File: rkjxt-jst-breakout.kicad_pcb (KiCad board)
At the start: 2 copper layers, 34 x 26.8 mm, 8 parts

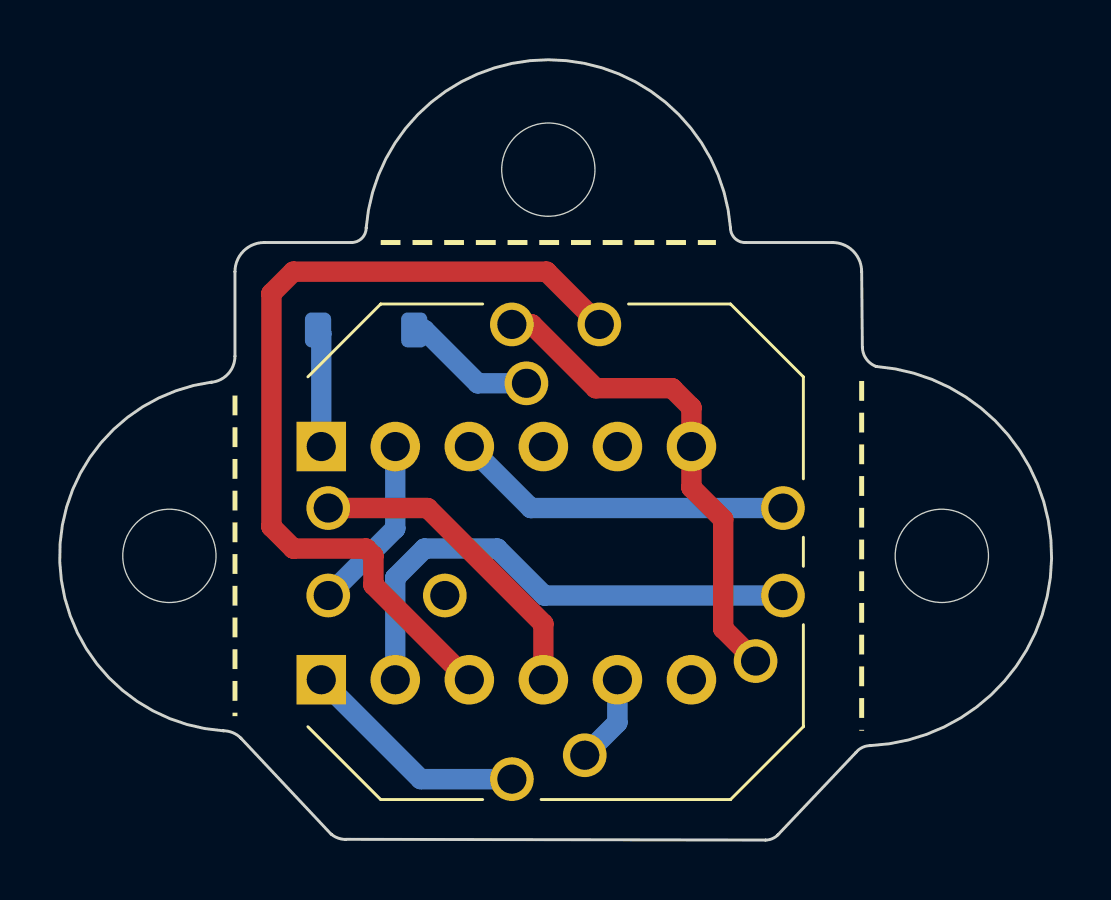
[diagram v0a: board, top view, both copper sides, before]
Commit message: fixing some issues, adding images
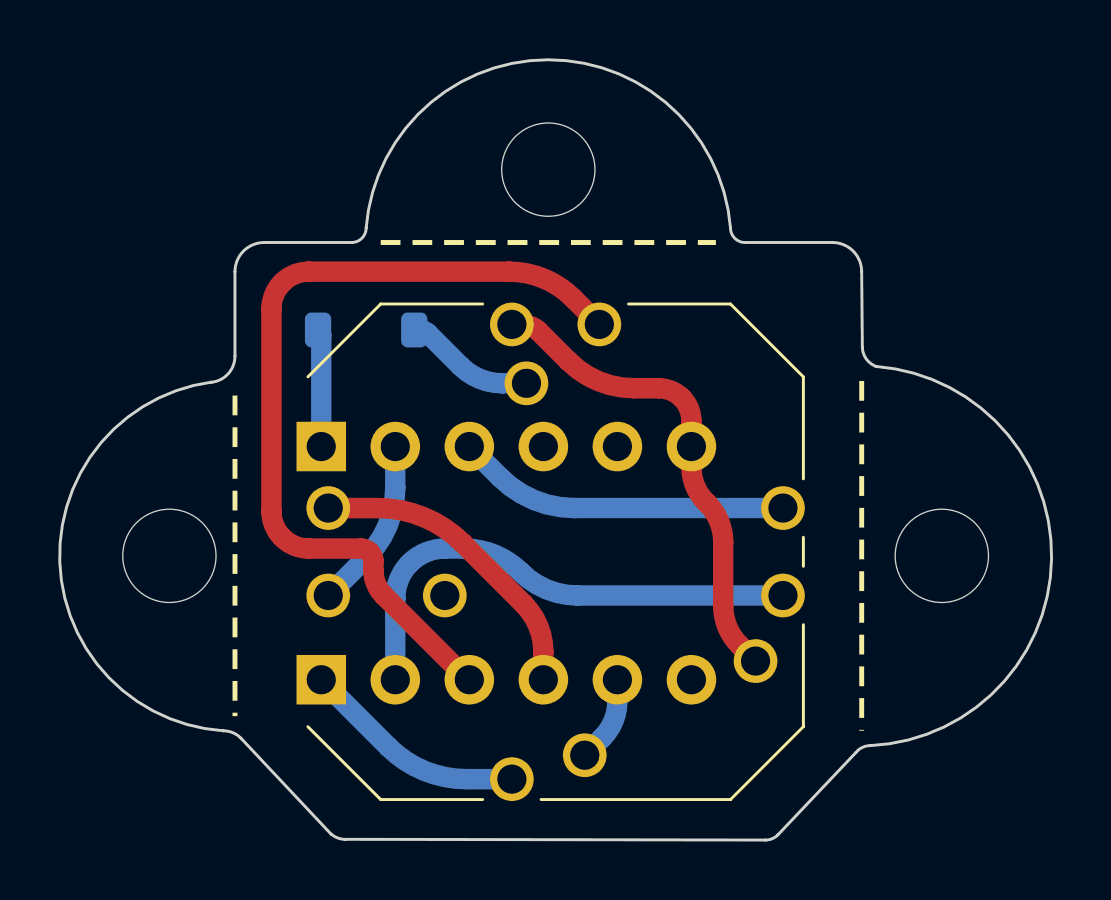
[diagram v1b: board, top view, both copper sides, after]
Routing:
- net Gnd: track 17.0 -> 16.4 mm
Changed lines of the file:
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@@
       (effects (font (size 1 1) (thickness 0.17) bold) (justify left top))
   )
-  (segment (start 134.96 75.11) (end 134.96 79) (width 0.7) (layer "B.Cu") (net 4))
-  (segment (start 134.85 75) (end 134.96 75.11) (width 0.7) (layer "B.Cu") (net 4))
-  (segment (start 140.33 76.83) (end 138.5 75) (width 0.7) (layer "B.Cu") (net 5))
-  (segment (start 138.5 75) (end 138.15 75) (width 0.7) (layer "B.Cu") (net 5))
-  (segment (start 142 76.83) (end 140.33 76.83) (width 0.7) (layer "B.Cu") (net 5))
-  (segment (start 145.12 88.47) (end 145.12 87) (width 0.7) (layer "B.Cu") (net 6))
-  (segment (start 144 89.59) (end 145.12 88.47) (width 0.7) (layer "B.Cu") (net 6))
-  (segment (start 142.58 85.08) (end 142.58 87) (width 0.7) (layer "F.Cu") (net 7))
-  (segment (start 138.61 81.11) (end 142.58 85.08) (width 0.7) (layer "F.Cu") (net 7))
-  (segment (start 135.2 81.11) (end 138.61 81.11) (width 0.7) (layer "F.Cu") (net 7))
-  (segment (start 133.25 81.75) (end 134 82.5) (width 0.7) (layer "F.Cu") (net 8))
-  (segment (start 144.5 74.81) (end 142.69 73) (width 0.7) (layer "F.Cu") (net 8))
-  (segment (start 134 73) (end 133.25 73.75) (width 0.7) (layer "F.Cu") (net 8))
-  (segment (start 136.75 83.75) (end 140 87) (width 0.7) (layer "F.Cu") (net 8))
-  (segment (start 136.5 82.5) (end 136.75 82.75) (width 0.7) (layer "F.Cu") (net 8))
-  (segment (start 133.25 73.75) (end 133.25 81.75) (width 0.7) (layer "F.Cu") (net 8))
-  (segment (start 142.69 73) (end 134 73) (width 0.7) (layer "F.Cu") (net 8))
-  (segment (start 136.75 82.75) (end 136.75 83.75) (width 0.7) (layer "F.Cu") (net 8))
-  (segment (start 134 82.5) (end 136.5 82.5) (width 0.7) (layer "F.Cu") (net 8))
-  (segment (start 140 87) (end 140.04 87) (width 0.7) (layer "F.Cu") (net 8))
-  (segment (start 138.5 82.5) (end 137.5 83.5) (width 0.7) (layer "B.Cu") (net 9))
-  (segment (start 137.5 83.5) (end 137.5 87) (width 0.7) (layer "B.Cu") (net 9))
-  (segment (start 141 82.5) (end 138.5 82.5) (width 0.7) (layer "B.Cu") (net 9))
-  (segment (start 150.8 84.11) (end 142.61 84.11) (width 0.7) (layer "B.Cu") (net 9))
-  (segment (start 142.61 84.11) (end 141 82.5) (width 0.7) (layer "B.Cu") (net 9))
-  (segment (start 141.5 90.41) (end 138.37 90.41) (width 0.7) (layer "B.Cu") (net 10))
-  (segment (start 138.37 90.41) (end 134.96 87) (width 0.7) (layer "B.Cu") (net 10))
-  (segment (start 137.5 81.81) (end 135.2 84.11) (width 0.7) (layer "B.Cu") (net 11))
-  (segment (start 137.5 79) (end 137.5 81.81) (width 0.7) (layer "B.Cu") (net 11))
-  (segment (start 142.15 81.11) (end 140.04 79) (width 0.7) (layer "B.Cu") (net 12))
-  (segment (start 150.8 81.11) (end 142.15 81.11) (width 0.7) (layer "B.Cu") (net 12))
-  (segment (start 147 77) (end 144.375 77) (width 0.7) (layer "F.Cu") (net 13))
-  (segment (start 147.66 77.66) (end 147 77) (width 0.7) (layer "F.Cu") (net 13))
-  (segment (start 142.185 74.81) (end 141.5 74.81) (width 0.7) (layer "F.Cu") (net 13))
-  (segment (start 147.66 80.41) (end 147.66 79) (width 0.7) (layer "F.Cu") (net 13))
-  (segment (start 147.66 79) (end 147.66 77.66) (width 0.7) (layer "F.Cu") (net 13))
-  (segment (start 149.86 86.36) (end 148.75 85.25) (width 0.7) (layer "F.Cu") (net 13))
-  (segment (start 148.75 85.25) (end 148.75 81.5) (width 0.7) (layer "F.Cu") (net 13))
-  (segment (start 148.75 81.5) (end 147.66 80.41) (width 0.7) (layer "F.Cu") (net 13))
-  (segment (start 144.375 77) (end 142.185 74.81) (width 0.7) (layer "F.Cu") (net 13))
+  (segment (start 134.96 75.187781) (end 134.96 79) (width 0.7) (layer "B.Cu") (net 4))
+  (segment (start 134.905 75.055) (end 134.85 75) (width 0.7) (layer "B.Cu") (net 4))
+  (arc (start 134.905 75.055) (mid 134.945705 75.11592) (end 134.96 75.187781) (width 0.7) (layer "B.Cu") (net 4))
+  (segment (start 138.623743 75.123743) (end 139.739565 76.239565) (width 0.7) (layer "B.Cu") (net 5))
+  (segment (start 138.325 75) (end 138.15 75) (width 0.7) (layer "B.Cu") (net 5))
+  (segment (start 141.165 76.83) (end 142 76.83) (width 0.7) (layer "B.Cu") (net 5))
+  (arc (start 139.739565 76.239565) (mid 140.39356 76.67655) (end 141.165 76.83) (width 0.7) (layer "B.Cu") (net 5))
+  (arc (start 138.623743 75.123743) (mid 138.486678 75.032159) (end 138.325 75) (width 0.7) (layer "B.Cu") (net 5))
+  (segment (start 145.12 87.735) (end 145.12 87) (width 0.7) (layer "B.Cu") (net 6))
+  (segment (start 144.600276 88.989723) (end 144 89.59) (width 0.7) (layer "B.Cu") (net 6))
+  (arc (start 145.12 87.735) (mid 144.984928 88.414051) (end 144.600276 88.989723) (width 0.7) (layer "B.Cu") (net 6))
+  (segment (start 142.58 86.04) (end 142.58 87) (width 0.7) (layer "F.Cu") (net 7))
+  (segment (start 141.901177 84.401177) (end 139.815617 82.315617) (width 0.7) (layer "F.Cu") (net 7))
+  (segment (start 136.905 81.11) (end 135.2 81.11) (width 0.7) (layer "F.Cu") (net 7))
+  (arc (start 139.815617 82.315617) (mid 138.480214 81.423329) (end 136.905 81.11) (width 0.7) (layer "F.Cu") (net 7))
+  (arc (start 141.901177 84.401177) (mid 142.403579 85.153075) (end 142.58 86.04) (width 0.7) (layer "F.Cu") (net 7))
+  (segment (start 143.595 73.905) (end 144.5 74.81) (width 0.7) (layer "F.Cu") (net 8))
+  (segment (start 137.103553 84.103553) (end 139.985857 86.985857) (width 0.7) (layer "F.Cu") (net 8))
+  (segment (start 133.25 81.219669) (end 133.25 74.28033) (width 0.7) (layer "F.Cu") (net 8))
+  (segment (start 141.410136 73) (end 134.53033 73) (width 0.7) (layer "F.Cu") (net 8))
+  (segment (start 136.75 83.25) (end 136.75 82.926776) (width 0.7) (layer "F.Cu") (net 8))
+  (segment (start 136.323223 82.5) (end 134.53033 82.5) (width 0.7) (layer "F.Cu") (net 8))
+  (segment (start 140.02 87) (end 140.04 87) (width 0.7) (layer "F.Cu") (net 8))
+  (arc (start 136.625 82.625) (mid 136.717513 82.763456) (end 136.75 82.926776) (width 0.7) (layer "F.Cu") (net 8))
+  (arc (start 143.595 73.905) (mid 142.592576 73.235201) (end 141.410136 73) (width 0.7) (layer "F.Cu") (net 8))
+  (arc (start 136.75 83.25) (mid 136.841885 83.711939) (end 137.103553 84.103553) (width 0.7) (layer "F.Cu") (net 8))
+  (arc (start 133.25 81.219669) (mid 133.347459 81.70963) (end 133.625 82.125) (width 0.7) (layer "F.Cu") (net 8))
+  (arc (start 139.985857 86.985857) (mid 140.001522 86.996324) (end 140.02 87) (width 0.7) (layer "F.Cu") (net 8))
+  (arc (start 134.53033 73) (mid 134.040368 73.097459) (end 133.625 73.375) (width 0.7) (layer "F.Cu") (net 8))
+  (arc (start 133.625 82.125) (mid 134.040368 82.40254) (end 134.53033 82.5) (width 0.7) (layer "F.Cu") (net 8))
+  (arc (start 136.625 82.625) (mid 136.486543 82.532486) (end 136.323223 82.5) (width 0.7) (layer "F.Cu") (net 8))
+  (arc (start 133.625 73.375) (mid 133.347459 73.790368) (end 133.25 74.28033) (width 0.7) (layer "F.Cu") (net 8))
+  (segment (start 137.5 84.207106) (end 137.5 87) (width 0.7) (layer "B.Cu") (net 9))
+  (segment (start 139.861558 82.5) (end 139.207106 82.5) (width 0.7) (layer "B.Cu") (net 9))
+  (segment (start 143.748441 84.11) (end 150.8 84.11) (width 0.7) (layer "B.Cu") (net 9))
+  (arc (start 141.805 83.305) (mid 140.913341 82.709212) (end 139.861558 82.5) (width 0.7) (layer "B.Cu") (net 9))
+  (arc (start 139.207106 82.5) (mid 138.553825 82.629945) (end 138 83) (width 0.7) (layer "B.Cu") (net 9))
+  (arc (start 141.805 83.305) (mid 142.696658 83.900787) (end 143.748441 84.11) (width 0.7) (layer "B.Cu") (net 9))
+  (arc (start 138 83) (mid 137.629945 83.553825) (end 137.5 84.207106) (width 0.7) (layer "B.Cu") (net 9))
+  (segment (start 139.935 90.41) (end 141.5 90.41) (width 0.7) (layer "B.Cu") (net 10))
+  (segment (start 137.263377 89.303377) (end 134.96 87) (width 0.7) (layer "B.Cu") (net 10))
+  (arc (start 137.263377 89.303377) (mid 138.489128 90.122398) (end 139.935 90.41) (width 0.7) (layer "B.Cu") (net 10))
+  (segment (start 136.506514 82.803485) (end 135.2 84.11) (width 0.7) (layer "B.Cu") (net 11))
+  (segment (start 137.5 80.405) (end 137.5 79) (width 0.7) (layer "B.Cu") (net 11))
+  (arc (start 137.5 80.405) (mid 137.241801 81.70305) (end 136.506514 82.803485) (width 0.7) (layer "B.Cu") (net 11))
+  (segment (start 141.095 80.055) (end 140.04 79) (width 0.7) (layer "B.Cu") (net 12))
+  (segment (start 143.641995 81.11) (end 150.8 81.11) (width 0.7) (layer "B.Cu") (net 12))
+  (arc (start 141.095 80.055) (mid 142.263571 80.835814) (end 143.641995 81.11) (width 0.7) (layer "B.Cu") (net 12))
+  (segment (start 145.6875 77) (end 146.533309 77) (width 0.7) (layer "F.Cu") (net 13))
+  (segment (start 141.8425 74.81) (end 141.5 74.81) (width 0.7) (layer "F.Cu") (net 13))
+  (segment (start 147.66 79.705) (end 147.66 79) (width 0.7) (layer "F.Cu") (net 13))
+  (segment (start 147.66 78.12669) (end 147.66 79) (width 0.7) (layer "F.Cu") (net 13))
+  (segment (start 149.305 85.805) (end 149.86 86.36) (width 0.7) (layer "F.Cu") (net 13))
+  (segment (start 148.75 82.270746) (end 148.75 84.465111) (width 0.7) (layer "F.Cu") (net 13))
+  (segment (start 148.205 80.955) (end 148.15851 80.90851) (width 0.7) (layer "F.Cu") (net 13))
+  (segment (start 143.446922 76.071922) (end 142.427184 75.052184) (width 0.7) (layer "F.Cu") (net 13))
+  (arc (start 143.446922 76.071922) (mid 144.474908 76.7588) (end 145.6875 77) (width 0.7) (layer "F.Cu") (net 13))
+  (arc (start 147.33 77.33) (mid 146.964475 77.085764) (end 146.533309 77) (width 0.7) (layer "F.Cu") (net 13))
+  (arc (start 147.33 77.33) (mid 147.574235 77.695524) (end 147.66 78.12669) (width 0.7) (layer "F.Cu") (net 13))
+  (arc (start 147.66 79.705) (mid 147.789558 80.356334) (end 148.15851 80.90851) (width 0.7) (layer "F.Cu") (net 13))
+  (arc (start 148.75 84.465111) (mid 148.894239 85.190253) (end 149.305 85.805) (width 0.7) (layer "F.Cu") (net 13))
+  (arc (start 142.427184 75.052184) (mid 142.158928 74.872941) (end 141.8425 74.81) (width 0.7) (layer "F.Cu") (net 13))
+  (arc (start 148.205 80.955) (mid 148.608359 81.558669) (end 148.75 82.270746) (width 0.7) (layer "F.Cu") (net 13))
 )
